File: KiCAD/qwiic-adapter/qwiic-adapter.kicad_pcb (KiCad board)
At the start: 2 copper layers, 10.7 x 10.9 mm, 7 parts, among them J1 Conn_01x04_Female, J2 GVDC, J3 VGDC, J4 GVCD, J5 VGCD, J7 PAD, J8 Conn_01x04_Female

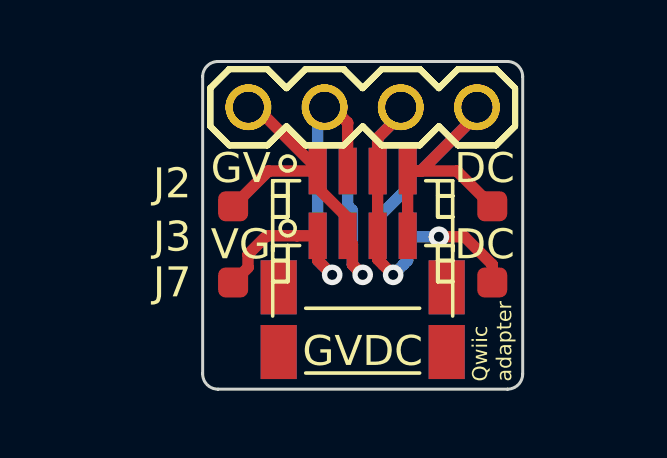
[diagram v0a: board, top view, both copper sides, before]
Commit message: qwiic adapter v0.9
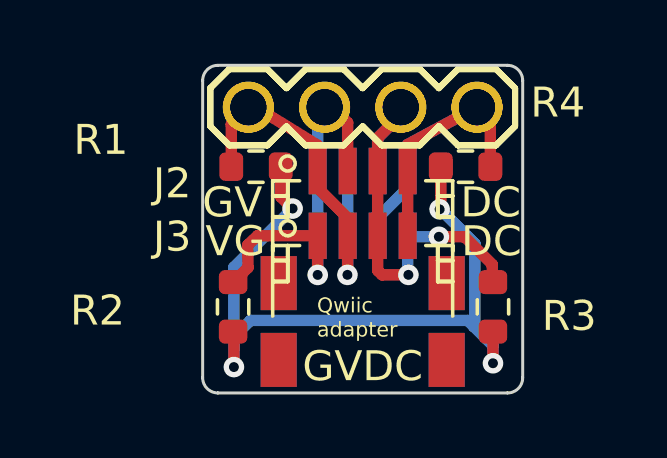
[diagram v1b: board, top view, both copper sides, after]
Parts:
- removed J7: PAD, library:PAD-4
- added R1: R, Resistor_SMD:R_0603_1608Metric, F.Cu at (139.7, 78.2)
- added R2: R, Resistor_SMD:R_0603_1608Metric, F.Cu at (138.9, 82.9)
- added R3: R, Resistor_SMD:R_0603_1608Metric, F.Cu at (147.6, 82.9)
- added R4: R, Resistor_SMD:R_0603_1608Metric, F.Cu at (146.7, 78.2)
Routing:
- net pull-up: track 0.00 -> 26.0 mm, vias 0 -> 4
- net GND0: track 13.9 -> 12.7 mm
- net GND2: track 15.1 -> 14.3 mm
- net GND3: track 14.1 -> 14.6 mm
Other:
- net class Default removed
- net class power removed
- board text added: "v0.9 2025 Oct 19"
- board text removed: "v0.5 2018 Dec 24"
